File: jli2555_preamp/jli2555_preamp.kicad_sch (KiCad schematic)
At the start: 25 parts, among them Q2 J113, U1 NMA0515SC, U2 NE5532

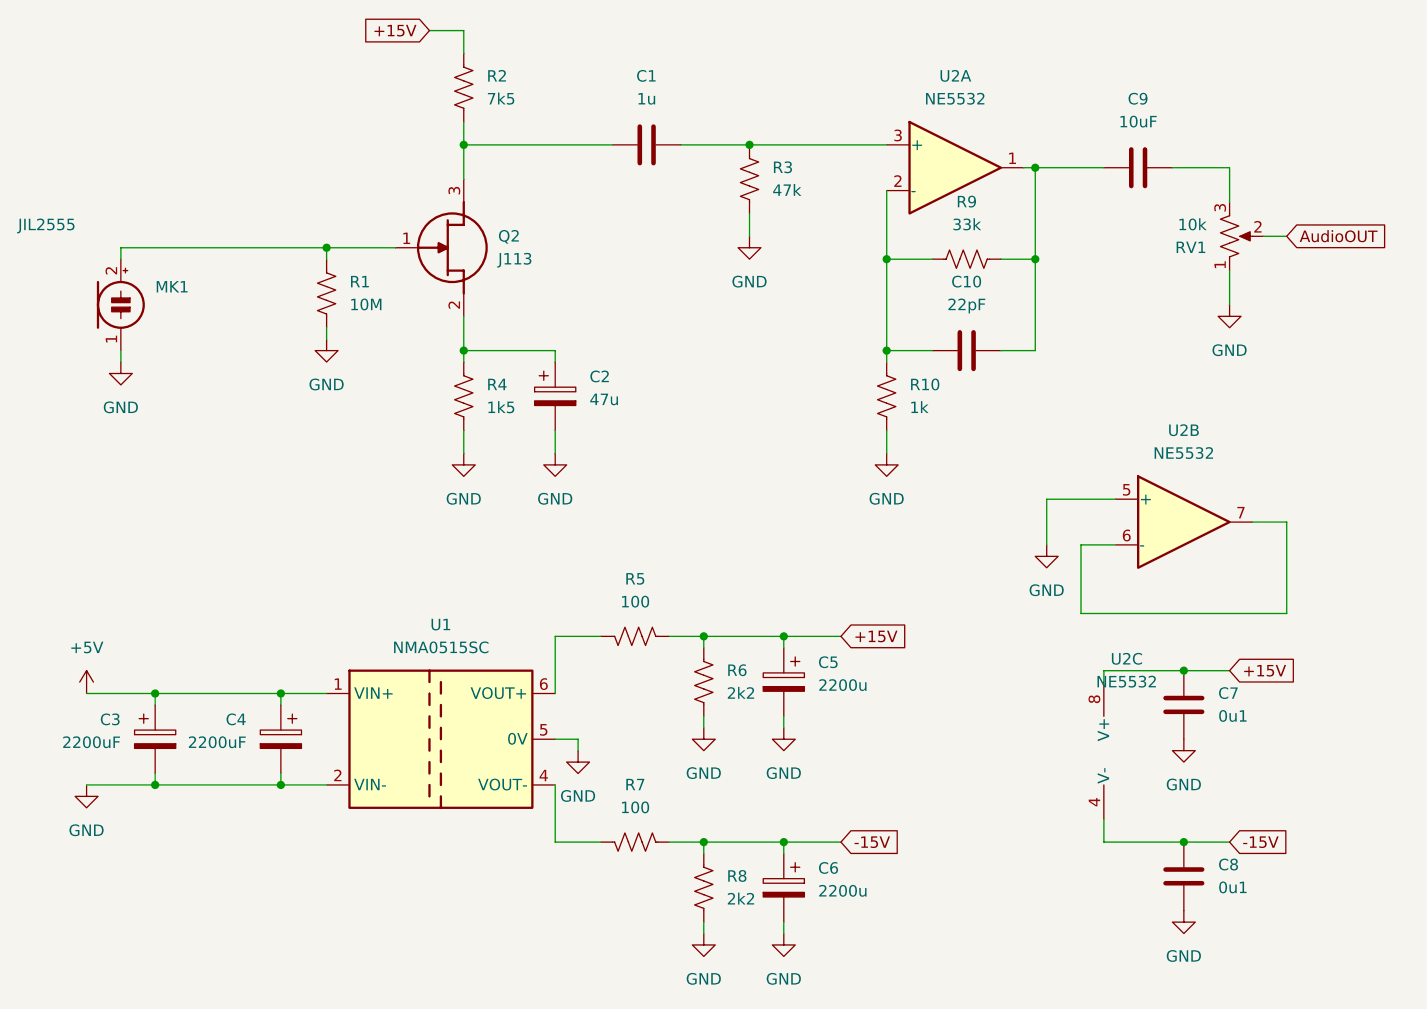
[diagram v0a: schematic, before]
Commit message: Finalize inital design of schematic
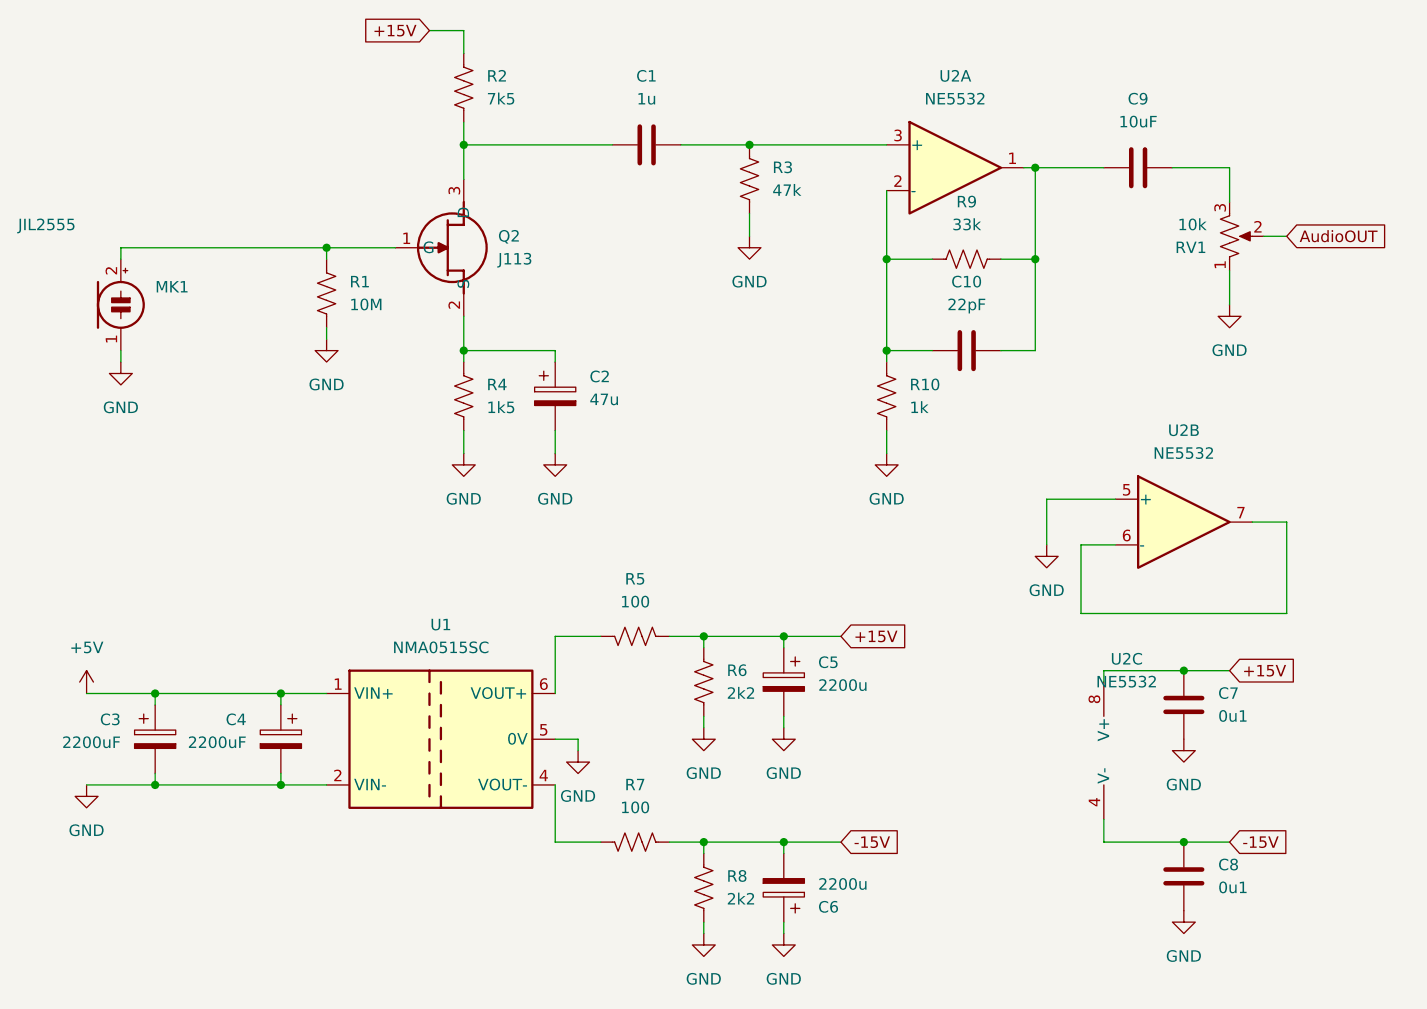
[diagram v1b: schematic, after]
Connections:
- net -15V: now also C6.2; no longer C6.1
- net GND: now also C6.1; no longer C6.2
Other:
- moved on the sheet: C6
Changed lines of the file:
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@@
 	(symbol
 		(lib_id "Device:C_Polarized")
-		(at 156.21 129.54 0)
-		(mirror y)
+		(at 156.21 129.54 180)
 		(unit 1)
 		(exclude_from_sim no)
@@
 		(on_board yes)
 		(dnp no)
-		(fields_autoplaced yes)
 		(property "Reference" "C6"
-			(at 160.02 127.3809 0)
+			(at 160.02 131.6991 0)
 			(effects
 				(font
@@
 		)
 		(property "Value" "2200u"
-			(at 160.02 129.9209 0)
+			(at 160.02 129.1591 0)
 			(effects
 				(font
@@
 		)
 		(property "Footprint" ""
-			(at 155.2448 133.35 0)
+			(at 155.2448 125.73 0)
 			(effects
 				(font
